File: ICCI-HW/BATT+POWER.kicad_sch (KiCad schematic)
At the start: 38 parts

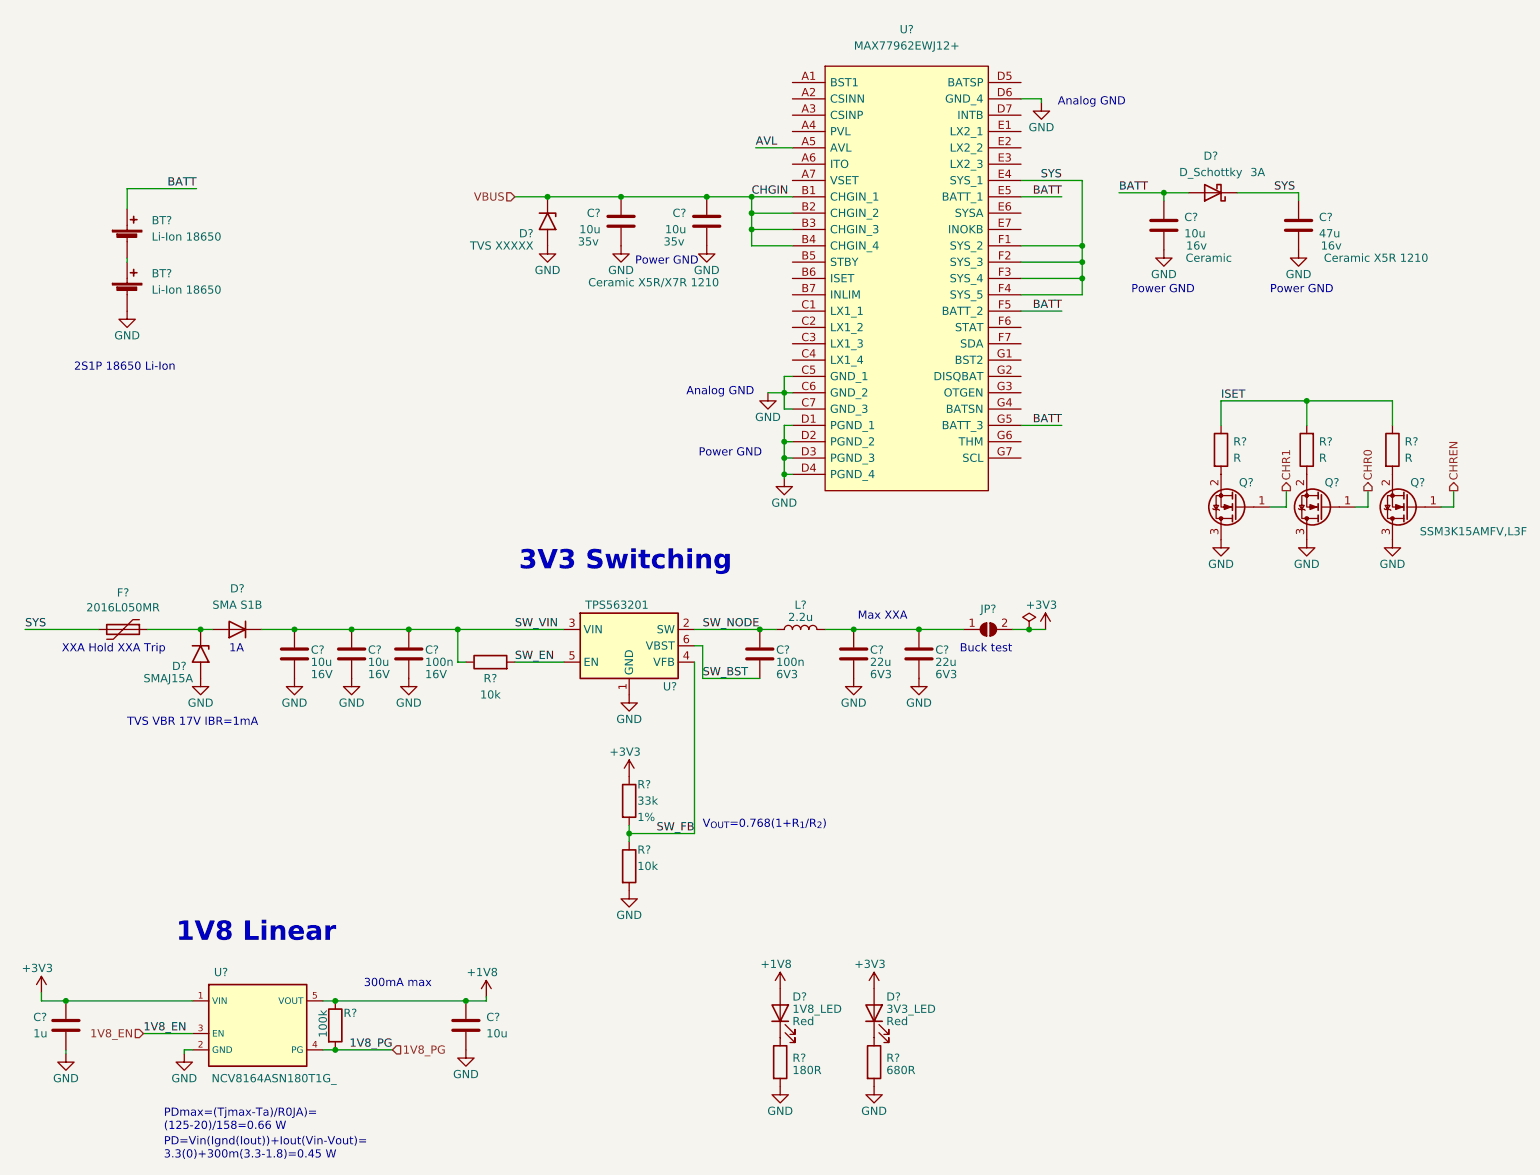
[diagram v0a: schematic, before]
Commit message: updated
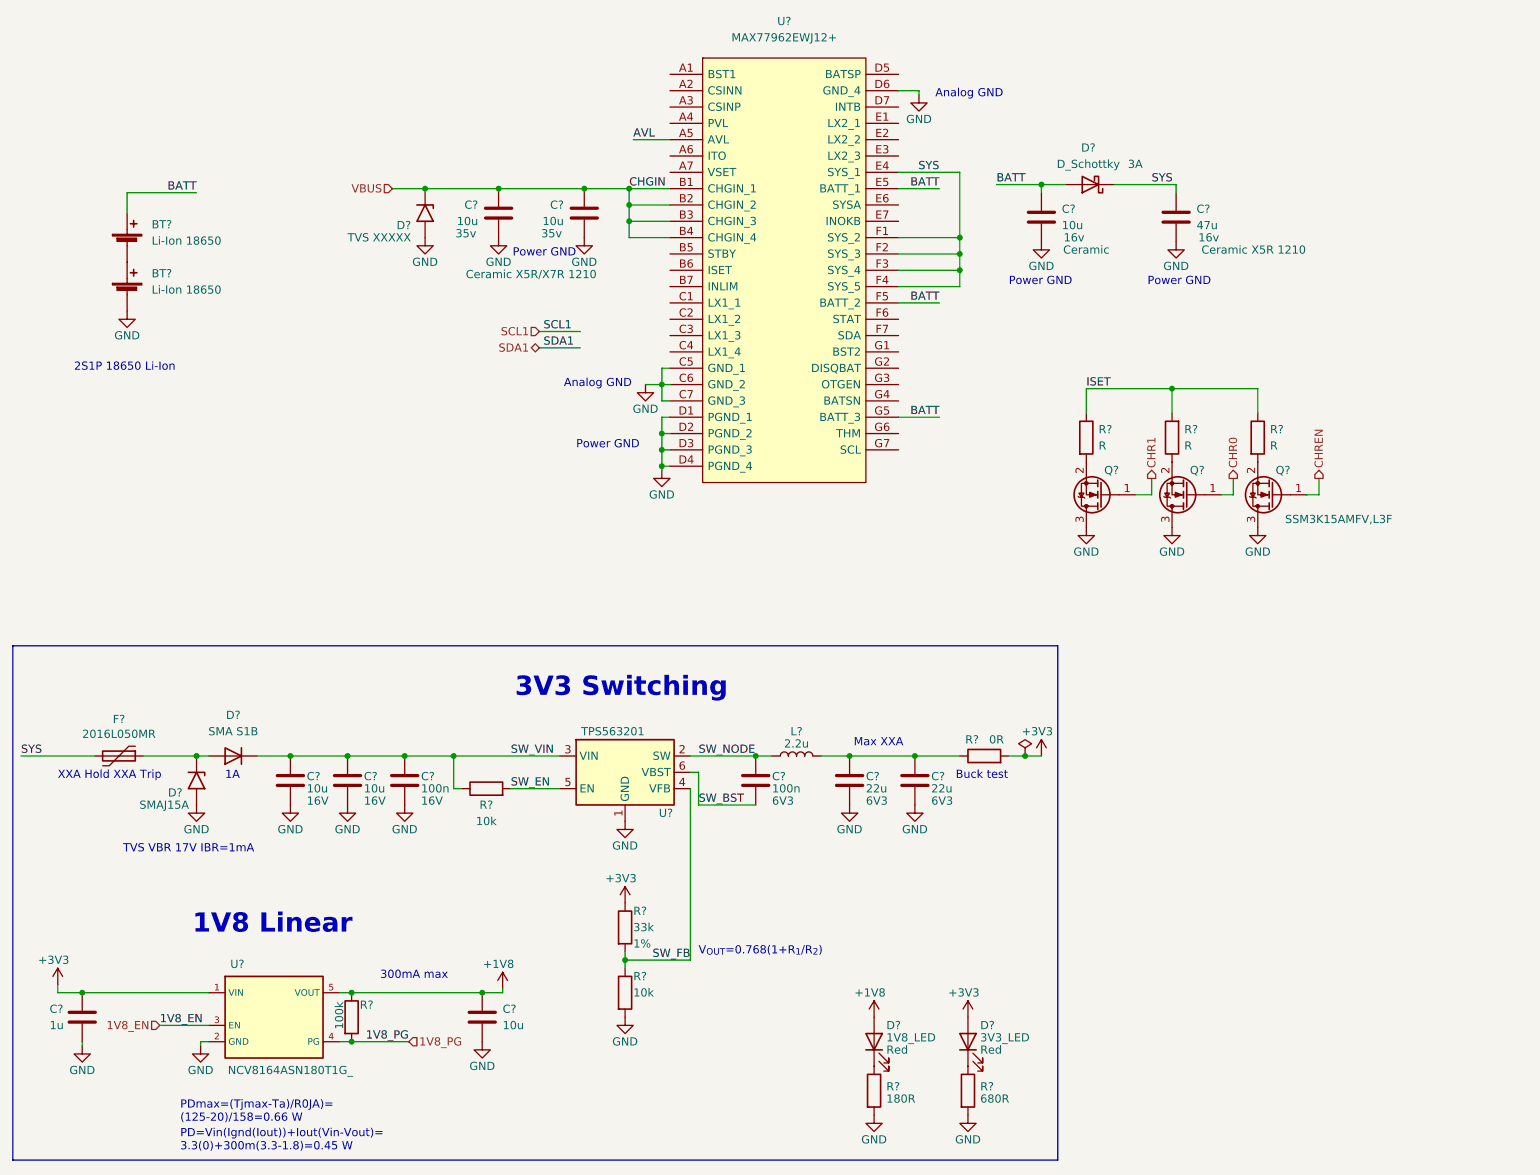
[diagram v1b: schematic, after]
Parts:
- removed JP?: SolderJumper_2_Open, symbol Jumper:SolderJumper_2_Open
- added R?: 0R, symbol Device:R
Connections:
- net +3V3: now also R?.2
- net at C?.1, C?.1, L?.2: now also R?.1
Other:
- moved on the sheet: BT?, C?, D?, F?, L?, Q?, R?, U?
